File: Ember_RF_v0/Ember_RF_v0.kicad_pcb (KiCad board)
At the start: 4 copper layers, 98.2 x 84.5 mm, 8 parts

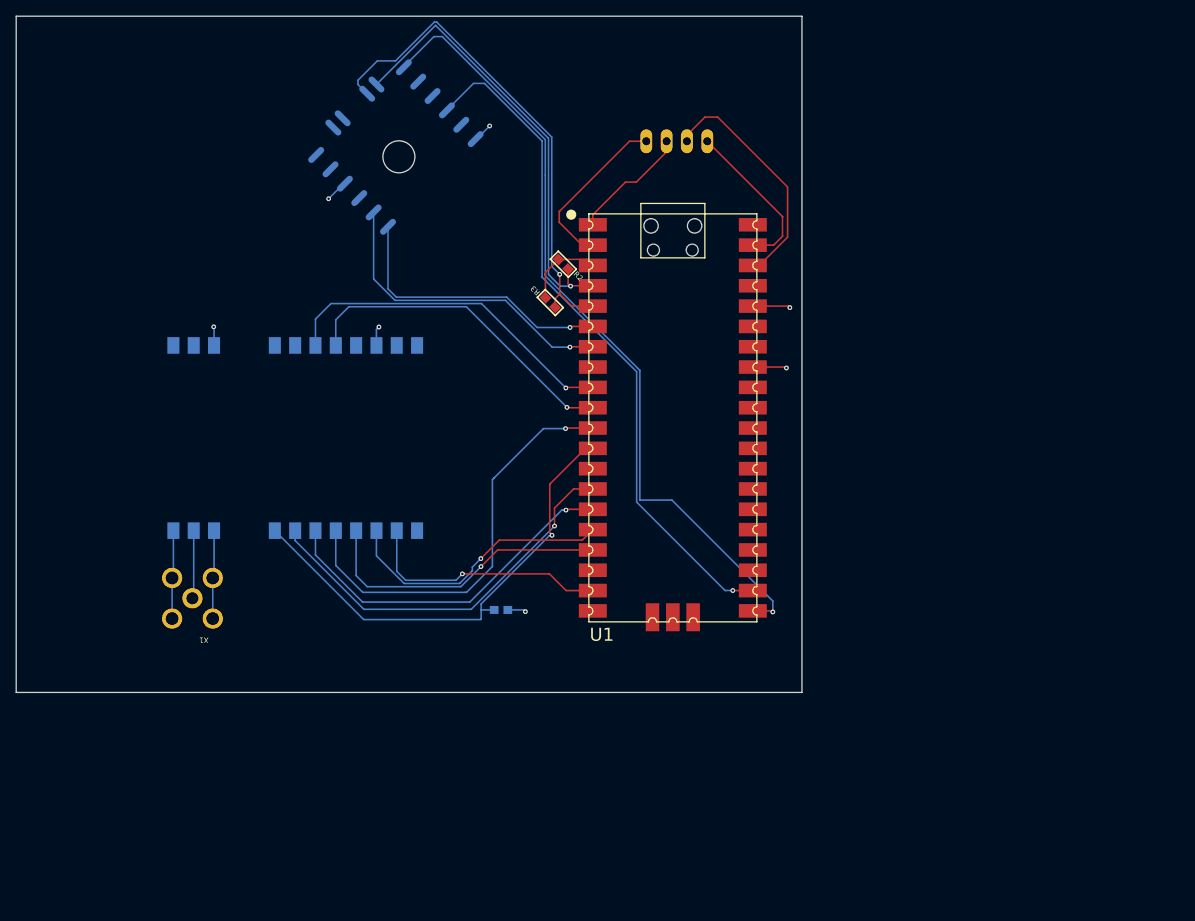
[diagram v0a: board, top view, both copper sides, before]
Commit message: All routings completed, Lisan Al-gaib!
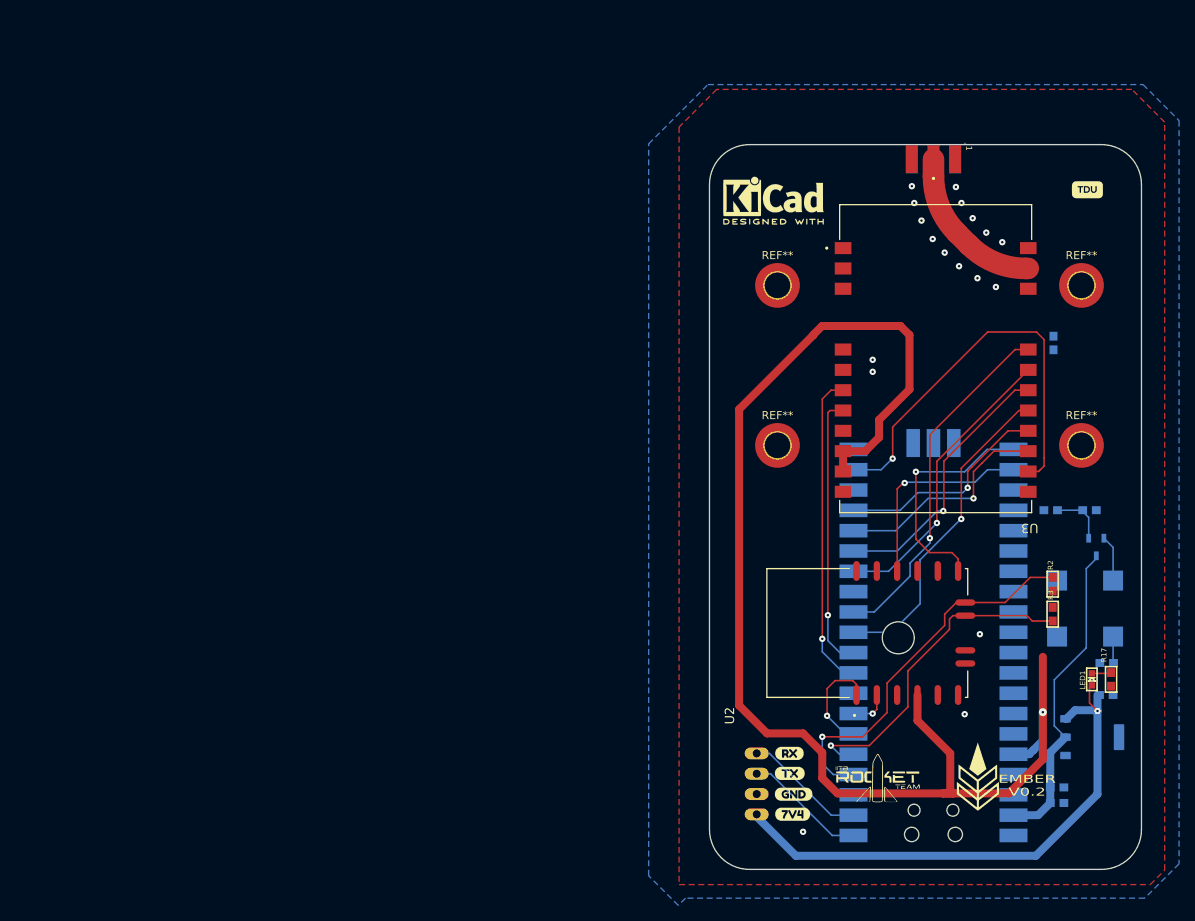
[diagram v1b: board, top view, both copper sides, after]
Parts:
- removed X1: ~, adafruit:SMA90_DIP
- added ?: , rx_label:RX0, F.Cu at (142.1, 116.5)
- added ?: , 7v4_label:7V40, F.Cu at (142.1, 124.1)
- added ?: , gnd_label:GND0, F.Cu at (142.1, 121.6)
- added ?: , tx_label:TX0, F.Cu at (142.1, 119.0)
- added C5: 10 uF, microbuilder:0603, B.Cu at (183.6, 109.2)
- added C6: 10 uF, microbuilder:0603, B.Cu at (177.4, 120.8)
- added C7: 10 uF, microbuilder:0603, B.Cu at (177.4, 122.7)
- added G***: LOGO, RT_Graphics:RT_logo, F.Cu at (155.0, 120.0)
- added G***: LOGO, RT_Graphics:TDU_label, F.Cu at (181.3, 46.1)
- added G***: LOGO, RT_Graphics:Ember_logo, F.Cu at (167.5, 119.5)
- added J1: ~, sma-connector:RFSOLUTIONS_CON-SMA-EDGE-S, F.Cu at (162.0, 42.2)
- added LED1: BATT_CONN, microbuilder:CHIPLED_0603, F.Cu at (181.8, 107.2)
- added LS2: BUZZER, CMT-8530S-SMT:CUI_CMT-8530S-SMT, B.Cu at (180.9, 98.4)
- added Q5: CJ3400, CJ3400:SOT95P240X115-3N, B.Cu at (182.3, 90.7)
- added R15: 100, microbuilder:0603, B.Cu at (183.7, 105.2)
- added R17: 100, microbuilder:0603, F.Cu at (184.2, 107.2)
- added R27: 1k, microbuilder:0603, B.Cu at (176.7, 86.1)
- added R4: 33k, microbuilder:0603, B.Cu at (181.5, 86.1)
- added REF**: KiCad-Logo2_5mm_SilkScreen, Symbol:KiCad-Logo2_5mm_SilkScreen, F.Cu at (142.0, 47.4)
- added REF**: MountingHole_3.2mm_M3_DIN965_Pad_TopOnly, MountingHole:MountingHole_3.2mm_M3_DIN965_Pad_TopOnly, F.Cu at (180.5, 78.0)
- added REF**: MountingHole_3.2mm_M3_DIN965_Pad_TopOnly, MountingHole:MountingHole_3.2mm_M3_DIN965_Pad_TopOnly, F.Cu at (142.5, 58.0)
- added REF**: MountingHole_3.2mm_M3_DIN965_Pad_TopOnly, MountingHole:MountingHole_3.2mm_M3_DIN965_Pad_TopOnly, F.Cu at (142.5, 78.0)
- added REF**: MountingHole_3.2mm_M3_DIN965_Pad_TopOnly, MountingHole:MountingHole_3.2mm_M3_DIN965_Pad_TopOnly, F.Cu at (180.5, 58.0)
- added U4: LDO Regulator 5v, AMS1117-5.0:SOT229P700X180-4N, B.Cu at (181.8, 114.5)
- U1: moved to B.Cu
- U2, U3: moved to F.Cu
- moved U3 82.1 mm to (162.3, 67.2), turned to 180 degrees
- moved JP2 80.9 mm to (139.9, 120.3), turned to 90 degrees
- moved U2 79.6 mm to (153.7, 101.5), turned to 90 degrees
- moved R1 76.7 mm to (177.0, 65.2), turned to -90 degrees
- moved R3 73.9 mm to (176.9, 99.1), turned to 90 degrees
- moved R2 73.1 mm to (176.9, 95.3), turned to 90 degrees
- moved U1 43.0 mm to (162.0, 102.6)
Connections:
- JP2 pad 1: /5V -> /V_BATT
- U1 pad P$24: unconnected-(U1-GP18-PadP$24) -> /BUZZER
- U1 pad P$39: /5V -> /5v
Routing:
- net /3v3: track 9.96 -> 167.6 mm, vias 3 -> 1
- net /GND: track 73.5 -> 0.00 mm, vias 4 -> 18
- net /GPS_WAKE_UP: track 100.4 -> 29.6 mm
- net /V_BATT: track 0.00 -> 68.7 mm, vias 0 -> 1
- net /GPS_RESET: track 85.4 -> 25.8 mm
- net /5v: track 0.00 -> 39.7 mm
- net /GPS_TX: track 39.3 -> 4.94 mm
- net /GPS_RX: track 35.4 -> 13.2 mm
- net /LORA_DIO1: track 31.3 -> 51.7 mm
- net /SCL: track 61.9 -> 41.7 mm
- net /5V: track 20.0 -> 0.00 mm
- net /LORA_CS: track 60.1 -> 44.3 mm
- net /LORA_SCK: track 49.6 -> 36.8 mm
- net /LORA_MISO: track 52.9 -> 40.3 mm
- net Net-(U3-ANT): track 8.52 -> 20.2 mm
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- added copper zone on B.Cu, net /GND
- added copper zone on F.Cu, net /GND
- removed copper zone on In1.Cu, net /3v3
- removed copper zone on In2.Cu, net /GND
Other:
- board size 98.2 x 84.5 mm -> 54 x 90.6 mm
- copper layers 4 -> 2
- board text added: "EMBER V0.2"
